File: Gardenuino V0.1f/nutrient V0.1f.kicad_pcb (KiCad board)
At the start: 2 copper layers, 99.1 x 71.1 mm, 86 parts, among them J1 Conn_01x04_Female, J10 Conn_01x01_Male, J2 Conn_01x04_Female, J3 Conn_01x04_Female, J4 Conn_01x04_Male, J5 Conn_01x04_Female, J6 Conn_01x04_Female, J7 Conn_01x03_Male, J8 Conn_01x03_Male, J9 Conn_01x01_Male, P1 SolderJumper_2_Bridged, P2 SolderJumper_2_Bridged, P3 SolderJumper_2_Bridged, P4 SolderJumper_2_Bridged, Q1 Q_NMOS_DGS, Q10 Q_NMOS_DGS, Q2 Q_NMOS_DGS, Q3 Q_NMOS_DGS, Q4 Q_NMOS_DGS, Q5 Q_NMOS_DGS, Q6 Q_NMOS_DGS, Q7 Q_NMOS_DGS, Q8 2N3904, U1 23LC512, U2 DS1307+, Y1 Crystal_Small

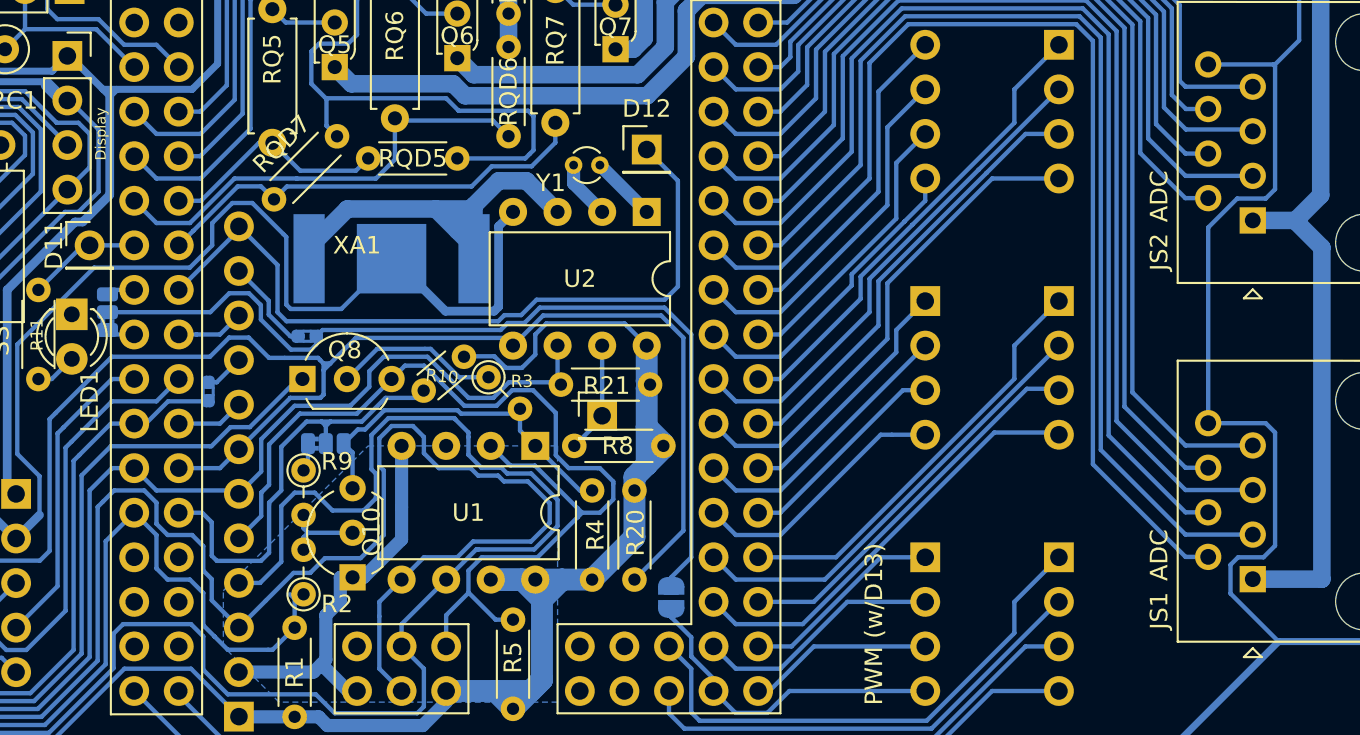
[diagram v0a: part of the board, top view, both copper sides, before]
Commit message: SpectDrone Development
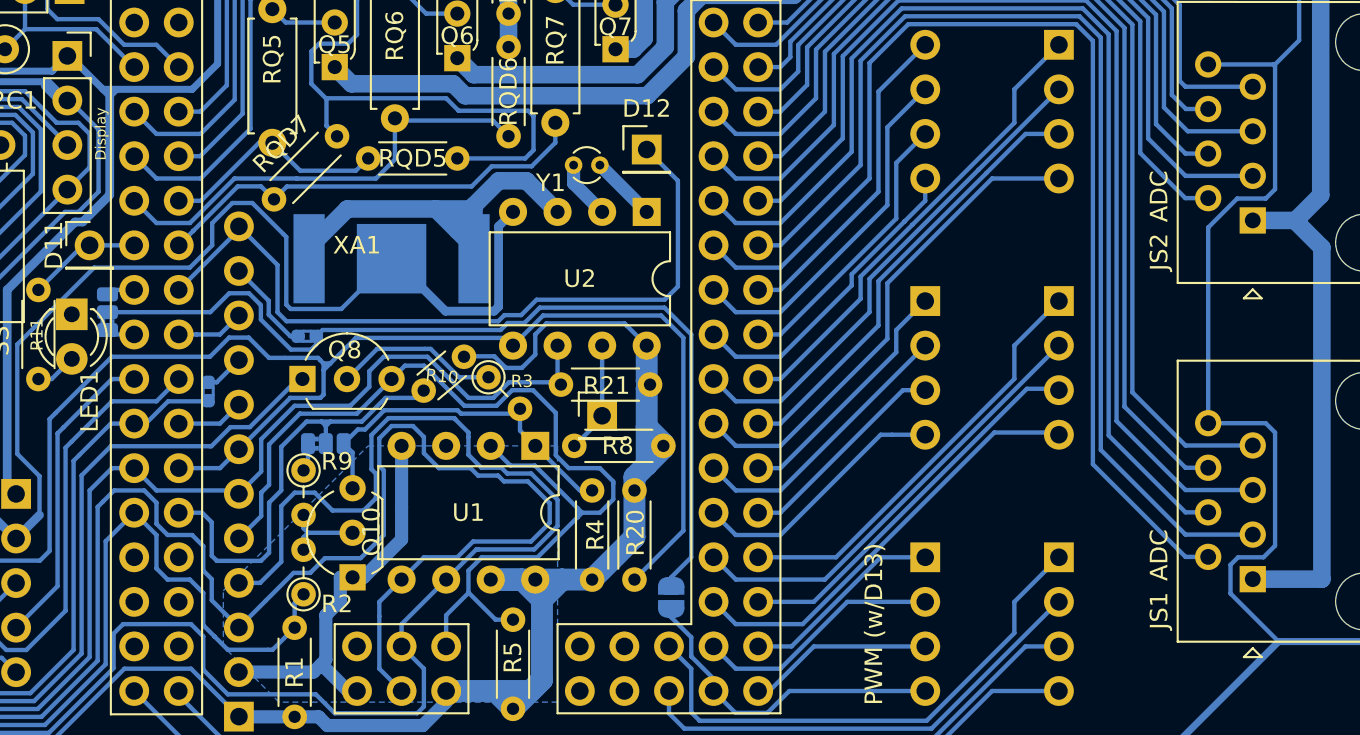
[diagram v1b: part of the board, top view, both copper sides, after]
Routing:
- net /RX1: track 25.8 -> 26.4 mm
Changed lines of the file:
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@@
     (fp_line (start 1.029025 -0.762) (end -1.029025 -0.762) (layer "B.SilkS") (width 0.12))
     (fp_line (start -2.0368 0) (end -2.3368 0.3) (layer "B.SilkS") (width 0.12))
-    (fp_arc (start -1.524 0.5588) (mid -1.750184 -0.279111) (end -1.029025 -0.762) (layer "B.SilkS") (width 0.12))
+    (fp_arc (start -1.524 0.5588) (mid -1.750184 -0.27911) (end -1.029025 -0.762) (layer "B.SilkS") (width 0.12))
     (fp_arc (start 1.029025 -0.762) (mid 1.750142 -0.279094) (end 1.524 0.5588) (layer "B.SilkS") (width 0.12))
     (fp_line (start 1.905 -0.889) (end -1.905 -0.889) (layer "B.CrtYd") (width 0.05))
@@
   (segment locked (start 164.737021 60.444913) (end 176.908935 60.444913) (width 0.25) (layer "B.Cu") (net 45))
   (segment locked (start 157.48 68.58) (end 158.75 68.58) (width 0.25) (layer "B.Cu") (net 45))
-  (segment locked (start 180.610106 68.342106) (end 181.864 69.596) (width 0.25) (layer "B.Cu") (net 46))
   (segment locked (start 180.610106 62.874649) (end 180.610106 68.342106) (width 0.25) (layer "B.Cu") (net 46))
   (segment locked (start 177.280348 59.544891) (end 180.610106 62.874649) (width 0.25) (layer "B.Cu") (net 46))
-  (segment locked (start 181.864 69.596) (end 185.568 69.596) (width 0.25) (layer "B.Cu") (net 46))
   (segment locked (start 164.364914 59.544891) (end 177.280348 59.544891) (width 0.25) (layer "B.Cu") (net 46))
-  (segment locked (start 185.568 69.596) (end 185.672 69.7) (width 0.25) (layer "B.Cu") (net 46))
   (segment locked (start 159.31648 64.593325) (end 164.364914 59.544891) (width 0.25) (layer "B.Cu") (net 46))
   (segment locked (start 157.48 66.04) (end 158.75 66.04) (width 0.25) (layer "B.Cu") (net 46))
   (segment locked (start 159.31648 65.47352) (end 159.31648 64.593325) (width 0.25) (layer "B.Cu") (net 46))
+  (segment (start 181.968 69.7) (end 185.672 69.7) (width 0.25) (layer "B.Cu") (net 46))
   (segment locked (start 158.75 66.04) (end 159.31648 65.47352) (width 0.25) (layer "B.Cu") (net 46))
+  (segment (start 180.610106 68.342106) (end 181.968 69.7) (width 0.25) (layer "B.Cu") (net 46))
   (segment locked (start 180.160095 69.289095) (end 180.160095 63.060355) (width 0.25) (layer "B.Cu") (net 47))
   (segment locked (start 159.766 64.779523) (end 159.766 66.294) (width 0.25) (layer "B.Cu") (net 47))
@@
   (segment (start 130.088 77.3195) (end 127.889 75.1205) (width 0.25) (layer "B.Cu") (net 67))
   (segment (start 143.975085 80.17848) (end 143.020502 80.17848) (width 0.25) (layer "B.Cu") (net 67))
-  (segment (start 124.460718 78.74) (end 127.889 75.311718) (width 0.25) (layer "B.Cu") (net 67))
   (segment locked (start 152.908 78.5495) (end 152.908 72.517) (width 0.25) (layer "B.Cu") (net 67))
   (segment locked (start 152.157524 79.299976) (end 152.908 78.5495) (width 0.25) (layer "B.Cu") (net 67))
+  (segment (start 127.889 75.311718) (end 127.889 75.1205) (width 0.25) (layer "B.Cu") (net 67))
+  (segment (start 124.460718 78.74) (end 127.889 75.311718) (width 0.25) (layer "B.Cu") (net 67))
   (segment locked (start 152.908 72.517) (end 151.13 70.739) (width 0.25) (layer "B.Cu") (net 67))
   (segment locked (start 110.363 63.373) (end 112.014 65.024) (width 0.25) (layer "B.Cu") (net 68))
@@
   (segment (start 129.5527 99.2505) (end 129.8067 99.2505) (width 0.25) (layer "B.Cu") (net 76))
   (segment locked (start 116.83232 103.53808) (end 112.171926 103.53808) (width 0.25) (layer "B.Cu") (net 76))
+  (segment (start 131.064 96.597) (end 131.572 96.089) (width 0.25) (layer "B.Cu") (net 76))
   (segment locked (start 127.254 99.2505) (end 129.5527 99.2505) (width 0.25) (layer "B.Cu") (net 76))
   (segment locked (start 110.923479 102.289633) (end 110.923479 73.861521) (width 0.25) (layer "B.Cu") (net 76))
   (segment locked (start 125.857 97.852782) (end 125.857 96.012) (width 0.25) (layer "B.Cu") (net 76))
+  (segment (start 131.064 97.9932) (end 131.064 96.597) (width 0.25) (layer "B.Cu") (net 76))
   (segment (start 129.8067 99.2505) (end 131.064 97.9932) (width 0.25) (layer "B.Cu") (net 76))
   (segment locked (start 110.923479 73.861521) (end 114.3 70.485) (width 0.25) (layer "B.Cu") (net 76))
@@
   (segment locked (start 120.2944 93.0656) (end 120.2944 100.076) (width 0.25) (layer "B.Cu") (net 76))
   (segment locked (start 126.492 98.4885) (end 127.254 99.2505) (width 0.25) (layer "B.Cu") (net 76))
-  (segment (start 131.064 97.9932) (end 131.064 96.343) (width 0.25) (layer "B.Cu") (net 76))
   (segment locked (start 125.857 96.012) (end 125.095 95.25) (width 0.25) (layer "B.Cu") (net 76))
-  (segment (start 131.064 96.343) (end 130.81 96.089) (width 0.25) (layer "B.Cu") (net 76))
   (segment locked (start 123.825 95.25) (end 125.095 95.25) (width 0.25) (layer "B.Cu") (net 76))
   (segment locked (start 148.59 85.9155) (end 148.59 81.915) (width 0.25) (layer "B.Cu") (net 77))
@@
   (segment locked (start 124.46 91.44) (end 125.7935 91.44) (width 0.25) (layer "B.Cu") (net 78))
   (segment (start 121.92 78.74) (end 120.65 78.74) (width 0.25) (layer "B.Cu") (net 79))
+  (segment (start 120.396 78.994) (end 120.65 78.74) (width 0.25) (layer "B.Cu") (net 79))
   (segment (start 152.14188 79.750469) (end 153.670001 81.27859) (width 0.25) (layer "B.Cu") (net 80))
   (segment (start 129.13848 80.42848) (end 130.8536 82.1436) (width 0.25) (layer "B.Cu") (net 80))
@@
   (segment locked (start 120.5865 86.36) (end 118.79344 88.15306) (width 0.25) (layer "B.Cu") (net 98))
   (segment locked (start 118.4656 88.4809) (end 118.4656 99.2632) (width 0.25) (layer "B.Cu") (net 98))
+  (segment (start 121.92 86.36) (end 122.5804 86.36) (width 0.25) (layer "B.Cu") (net 98))
   (segment (start 123.8504 85.09) (end 126.1026 85.09) (width 0.25) (layer "B.Cu") (net 98))
   (segment (start 122.5804 86.36) (end 123.8504 85.09) (width 0.25) (layer "B.Cu") (net 98))
@@
   (segment (start 125.476 81.28) (end 126.8095 81.28) (width 0.25) (layer "B.Cu") (net 99))
   (segment locked (start 124.46 81.28) (end 125.476 81.28) (width 0.25) (layer "B.Cu") (net 99))
+  (segment (start 120.396 81.026) (end 120.65 81.28) (width 0.25) (layer "B.Cu") (net 100))
   (segment (start 121.92 81.28) (end 120.65 81.28) (width 0.25) (layer "B.Cu") (net 100))
   (segment (start 129.588 79.3595) (end 127.889 77.6605) (width 0.25) (layer "B.Cu") (net 101))
